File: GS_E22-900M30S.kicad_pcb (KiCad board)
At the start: 2 copper layers, 60 x 60 mm, 11 parts, among them J1 Barrel_Jack, J3 Raspberry_Pi_2_3, U1 LT1085-5.0, U2 E22-900M30S

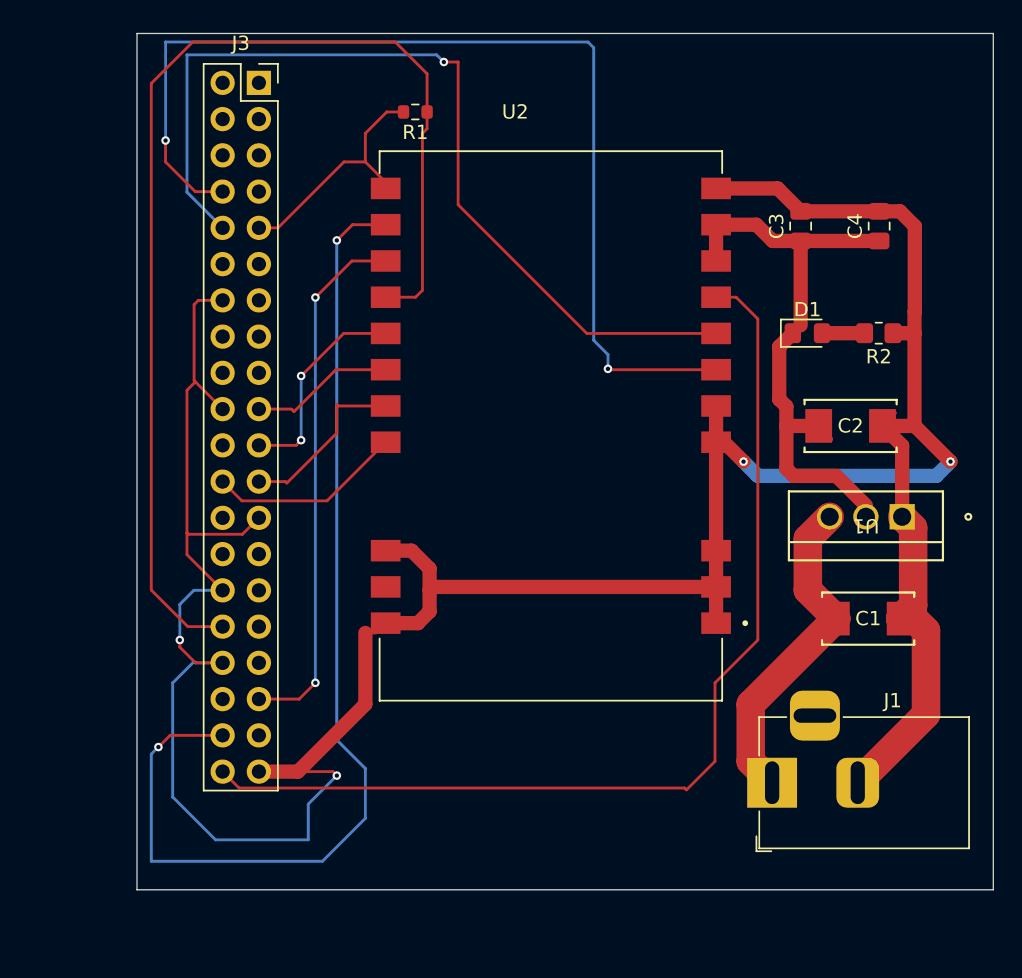
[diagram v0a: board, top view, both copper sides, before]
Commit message: Add files via upload
updated pcb
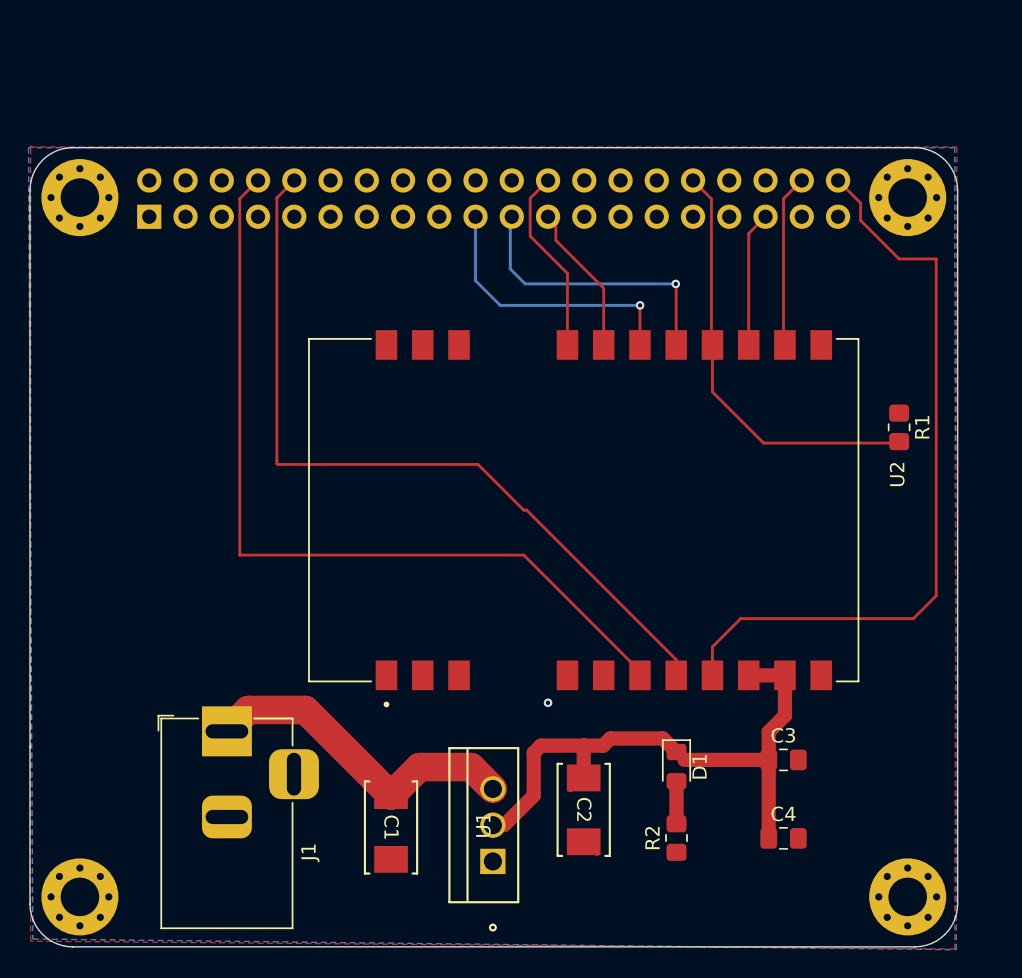
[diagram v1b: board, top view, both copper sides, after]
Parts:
- added G***: LOGO, LOGO, B.Cu at (97.5, 102.4)
- added H1: M, MountingHole:MountingHole_2.7mm_M2.5_Pad_Via, F.Cu at (82.0, 86.5)
- added H2: M, MountingHole:MountingHole_2.7mm_M2.5_Pad_Via, F.Cu at (140.0, 86.5)
- added H3: M, MountingHole:MountingHole_2.7mm_M2.5_Pad_Via, F.Cu at (82.0, 135.5)
- added H4: M, MountingHole:MountingHole_2.7mm_M2.5_Pad_Via, F.Cu at (140.0, 135.5)
- J3: moved to B.Cu
- R1: footprint Resistor_SMD:R_0603_1608Metric -> Resistor_SMD:R_0805_2012Metric_Pad1.20x1.40mm_HandSolder
- moved C4 43.4 mm to (131.3, 131.4), turned to 0 degrees
- moved R1 40.5 mm to (139.4, 102.6), turned to -90 degrees
- moved J1 38.4 mm to (92.3, 123.9), turned to 90 degrees
- moved R2 38.1 mm to (123.8, 131.4), turned to 90 degrees
- moved U1 37.5 mm to (110.9, 133.0), turned to 90 degrees
- moved C3 37.4 mm to (131.3, 125.9), turned to 0 degrees
- moved C1 36.5 mm to (103.8, 130.6), turned to -90 degrees
- moved C2 32.8 mm to (117.3, 129.4), turned to -90 degrees
- moved D1 31.7 mm to (123.8, 126.4), turned to -90 degrees
- moved J3 12.1 mm to (86.9, 87.8), turned to -90 degrees
- moved U2 6.33 mm to (117.3, 108.4), turned to -90 degrees
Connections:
- R1 pad 1: RF_RESET -> GND
- R1 pad 2: GND -> RF_RESET
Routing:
- net GND: track 237.9 -> 3.40 mm, vias 4 -> 1
- net RF_DIO1: track 74.5 -> 12.1 mm, vias 2 -> 0
- net RF_RESET: track 81.1 -> 30.0 mm
- net RF_BUSY: track 37.4 -> 9.47 mm, vias 2 -> 0
- net RF_DIO2: track 71.7 -> 52.6 mm
- net RF_RXEN: track 73.9 -> 58.5 mm, vias 2 -> 0
- net RF_MOSI: track 10.2 -> 19.5 mm, vias 0 -> 1
- net RF_TXEN: track 64.2 -> 55.1 mm, vias 1 -> 0
- net RF_MISO: track 14.8 -> 20.0 mm, vias 2 -> 1
- net RF_SCK: track 12.4 -> 10.6 mm
- net RF_CS: track 13.7 -> 13.1 mm
- added copper zone on B.Cu, net GND
- added copper zone on F.Cu, net GND
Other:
- board size 60 x 60 mm -> 65 x 56 mm
- board text added: "Argus-2 Ground Station"
- board text added: "Carnegie Mellon University"
